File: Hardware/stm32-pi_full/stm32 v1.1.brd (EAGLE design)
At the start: 131.4 x 105.8 mm, 287 parts, among them J1 JUMPER-SMT_2_NC_TRACE_NO-SILK, Q1 PNP, Q2 NPN, Q3 NPN, U1 ESP32-WROOM-32D

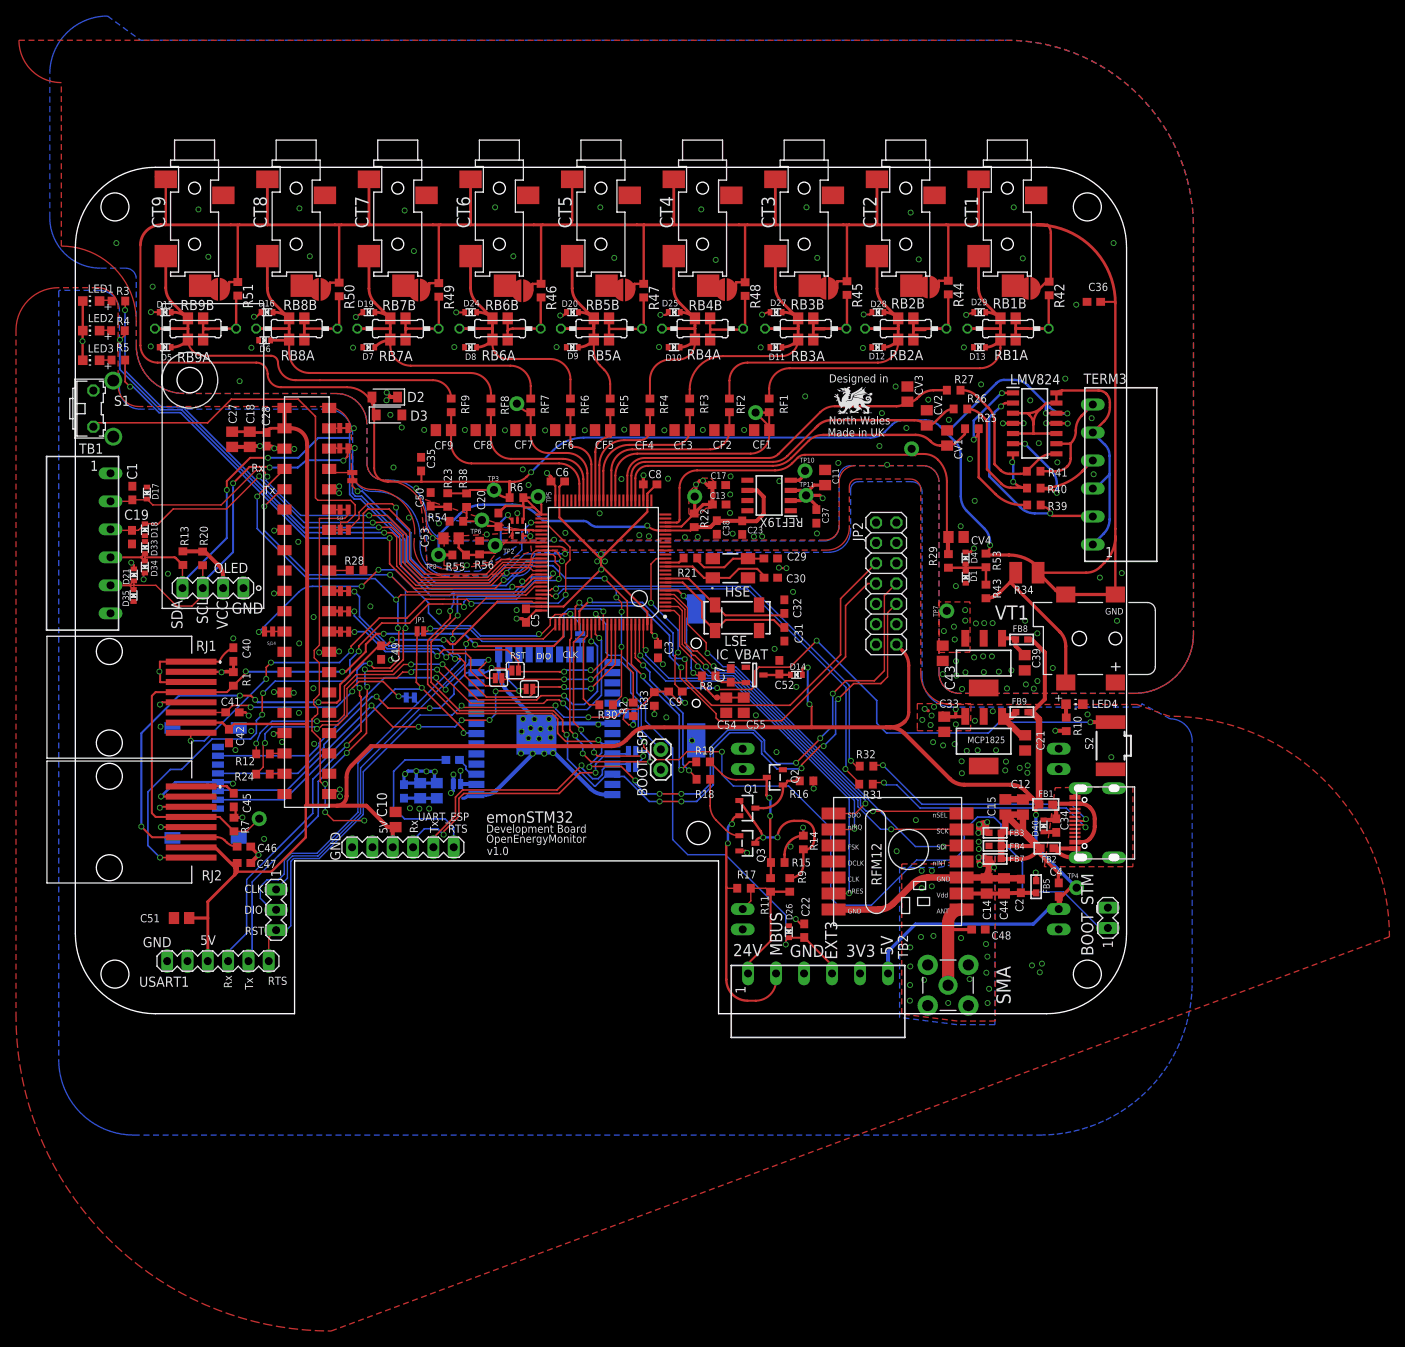
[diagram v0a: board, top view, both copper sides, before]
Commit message: tidy
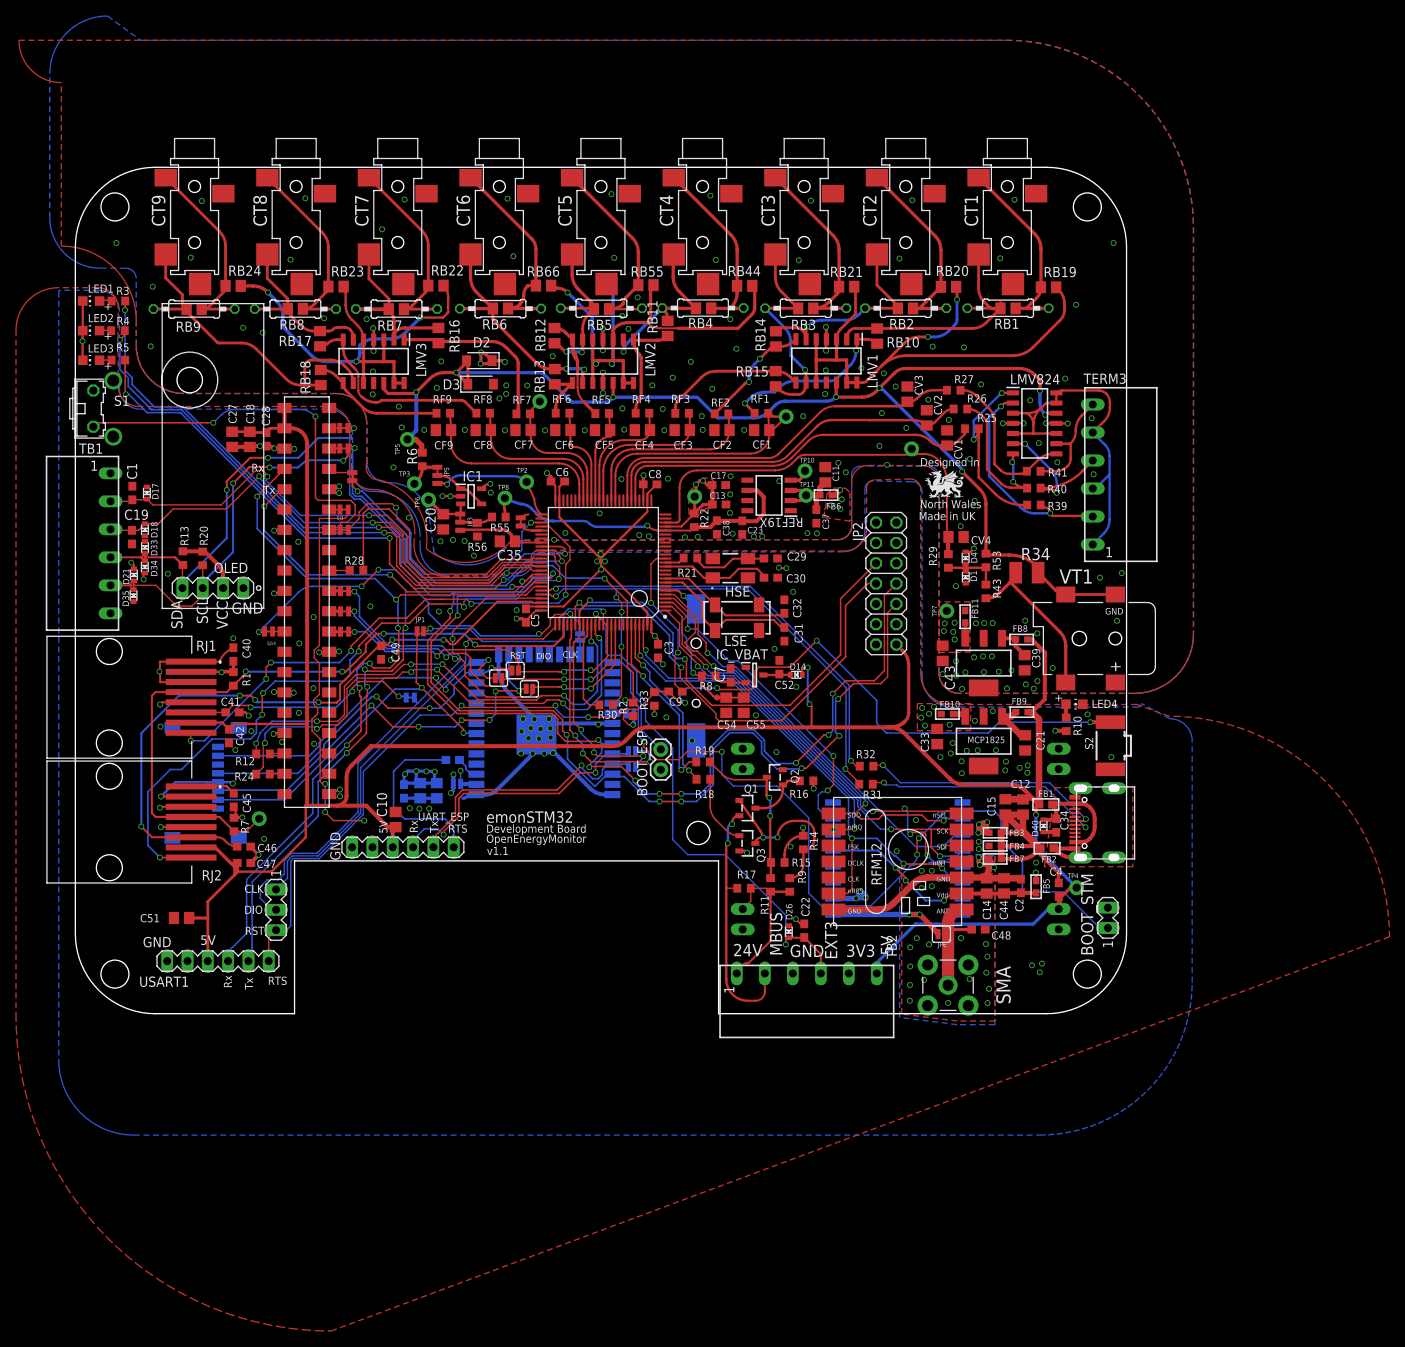
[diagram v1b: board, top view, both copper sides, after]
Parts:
- removed C36: (no value), rcl:C0603
- removed C50: 1uF, rcl:C0603
- removed C53: 22uF, rcl:C0805
- removed D10, D11, D12, D13, D15, D16, D19, D20, D24, D25, D27, D28, D29, D5, D6, D7, D8, D9: ESD5Z3.3T1G, microbuilder:SOD-523
- removed IC2: (no value), analog-devices:SC70-5
- removed JP10, JP11, JP12, JP13, JP14, JP15, JP16, JP17, JP18: JUMPER-SMT_2_NO_NO-SILK_ROUND, SparkFun-Jumpers:SMT-JUMPER_2_NO_NO-SILK_ROUND
- removed R23: 1k, resistor:R0603
- removed R38: 39k, resistor:R0603
- removed R42, R44, R45, R46, R47, R48, R49, R50, R51: 0R, rcl:R0603
- removed R54: 10k, resistor:R0603
- removed RB1A, RB2A, RB3A, RB4A, RB5A, RB6A, RB7A, RB8A, RB9A: 6R8, rcl:R0805
- removed RB1B, RB2B, RB3B, RB4B, RB5B, RB6B, RB7B, RB8B, RB9B: (no value), rcl:R0805
- added FB10, FB11, FB6: (no value), microbuilder:_0603
- added IC1: TS461CLT, TS461CLT:SOT95P280X145-5N
- added JP3, JP5: JUMPER-SMT_3_1-NC_TRACE_NO-SILK, SparkFun-Jumpers:SMT-JUMPER_3_1-NC_TRACE_NO-SILK
- added JP6: JUMPER-SMT_2_NC_PASTE_SILK, SparkFun-Jumpers:SMT-JUMPER_2_NC_PASTE_SILK
- added LMV1, LMV2, LMV3: LMV824IDG4, LMV824IDG4:SOIC127P600X175-14N
- added RB1, RB2, RB3, RB4, RB5, RB6, RB7, RB8, RB9: 6R81, rcl:R0805
- added RB10, RB11, RB12, RB13, RB14, RB15, RB16, RB17, RB18: 510R 0.1%, rcl:R0805
- added RB19, RB20, RB21, RB22, RB23, RB24, RB44, RB55, RB66: 680R | 681R 0.1%, rcl:R0805
- added SJ1: JUMPER-SMT_2_NC_TRACE_NO-SILK, SparkFun-Jumpers:SMT-JUMPER_2_NC_TRACE_NO-SILK
- added U2: RFM69HCW/RFM95W, microbuilder:RFMHCW_SMT
- C11, C23: value 1uF -> 22uf
- C20: value 2.2nF -> 22uF; device rcl:C0603 -> rcl:C0805
- C35: value (none) -> 22uF; device rcl:C0603 -> rcl:C0805
- FB1: value (none) -> 1600R
- FB2: value (none) -> 0R
- R55: value 91k -> 10k
- R6: value 0R -> 20R; device resistor:R0603 -> rcl:R0603
- moved TP5 17.8 mm to (41.5, 71.8)
- moved C35 14.5 mm to (54.0, 59.0), turned to 180 degrees
- moved R6 12.7 mm to (43.4, 69.3), turned to 90 degrees
- moved D2 12.7 mm to (50.5, 81.6)
- moved D3 12.1 mm to (50.7, 78.7)
- moved TP8 10.9 mm to (53.7, 64.5)
- moved TP3 9.98 mm to (42.4, 66.2)
- moved TP2 8.85 mm to (56.4, 66.5)
- moved TP6 7.12 mm to (44.2, 64.2)
- moved C20 6.90 mm to (46.0, 61.5), turned to 270 degrees
- moved R55 6.86 mm to (52.9, 62.1), turned to 0 degrees
- moved TP18 3.84 mm to (88.8, 74.6)
- moved TP19 2.88 mm to (58.1, 76.5)
- moved RB4_ 2.57 mm to (78.4, 88.2)
- moved RB1_ 2.54 mm to (116.6, 88.2)
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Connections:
- net CT1 renamed CT1_ADC
- net CT2 renamed CT2_ADC
- net CT3 renamed CT3_ADC
- net CT4 renamed CT4_ADC
- net CT5 renamed CT5_ADC
- net CT6 renamed CT6_ADC
- removed net OPAMP_NON-INVERT+: C53.1, IC2.3, R55.1, R56.2, STM32F303VE.58, TP2.1
- new net ANT_LORA: JP6.1, U2.1P
- new net BIAS123: LMV1.10, LMV1.13, LMV1.14, LMV1.3, LMV1.5, RB19.2, RB20.2, RB21.2
- new net BIAS456: LMV2.10, LMV2.13, LMV2.14, LMV2.3, LMV2.5, RB44.2, RB55.2, RB66.2
- new net BIAS789: LMV3.10, LMV3.13, LMV3.14, LMV3.3, LMV3.5, RB22.2, RB23.2, RB24.2
- new net BIAS_SOT23: IC1.1, IC1.4, JP5.2
- new net CT1_OUT: LMV1.1, RB10.1, RF1.1
- new net CT2_OUT: LMV1.7, RB14.1, RF2.1
- new net CT3_OUT: LMV1.8, RB15.2, RF3.1
- new net CT4_OUT: LMV2.1, RB11.1, RF4.1
- new net CT5_OUT: LMV2.7, RB12.1, RF5.1
- new net CT6_OUT: LMV2.8, RB13.2, RF6.1
- new net CT7_OUT: LMV3.1, RB16.1, RF7.1
- new net CT8_OUT: LMV3.7, RB17.1, RF8.1
- new net CT9_OUT: LMV3.8, RB18.2, RF9.1
- new net DIO1_RFM: STM32F303VE.3, U2.7P
- new net N$12: CT5.P$3
- new net N$38: CT4.P$3
- new net N$39: C20.1, IC1.3, JP3.3, TP6.1
- new net N$40: CT6.P$1, RB6.2, RB66.1, RB6_.2
- new net N$42: JP5.3, R6.1, TP3.1
- new net N$43: CT9.P$1, RB24.1, RB9.2, RB9_.2
- new net N$45: CT8.P$1, RB23.1, RB8.2, RB8_.2
- new net N$46: CT7.P$1, RB22.1, RB7.2, RB7_.2
- new net STM32_OPAMP_NON-INVERT+: C35.1, JP3.1, STM32F303VE.58
- new net STM32_OPAMP_OUT: JP5.1, STM32F303VE.51, TP2.1
- net +3V3: now also FB10.2; no longer MCP1825.3
- net +3V3ANA: now also FB11.2, FB6.2, IC1.2, LMV1.4, LMV2.4, LMV3.4; no longer C11.1, C37.1, D15.K, D16.K, D19.K, D20.K, D24.K, D25.K, D27.K, D28.K, D29.K, IC2.5, MCP1825(ANALOG).3, REF19X.2, REF19X.3, TP11.1
- net AGND: now also C20.2, IC1.5, LMV1.11, LMV2.11, LMV3.11; no longer C36.2, C50.2, C53.2, D10.A, D11.A, D12.A, D13.A, D5.A, D6.A, D7.A, D8.A, D9.A, IC2.2, R54.2
- net ANT: now also JP6.2
- net BIAS: now also LMV1.12, LMV2.12, LMV3.12, TP5.1; no longer C35.1, C36.1, CT1.P$1, CT2.P$1, CT3.P$1, CT4.P$1, CT5.P$1, CT6.P$1, CT7.P$1, CT8.P$1, CT9.P$1, JP10.1, JP11.1, JP12.1, JP13.1, JP14.1, JP15.1, JP16.1, JP17.1, JP18.1, R23.2, R38.1, R42.1, R44.1, R45.1, R46.1, R47.1, R48.1, R49.1, R50.1, R51.1, TP3.1
- net CT_IN1: now also LMV1.2, RB1.1, RB10.2; no longer D13.K, D29.A, RB1A.1, RB1B.1, RF1.1
- net CT_IN2: now also LMV1.6, RB14.2, RB2.1; no longer D12.K, D28.A, RB2A.1, RB2B.1, RF2.1
- net CT_IN3: now also LMV1.9, RB15.1, RB3.1; no longer D11.K, D27.A, RB3A.1, RB3B.1, RF3.1
- net CT_IN4: now also LMV2.2, RB11.2, RB4.1; no longer D10.K, D25.A, RB4A.1, RB4B.1, RF4.1
- net CT_IN5: now also LMV2.6, RB12.2, RB5.1; no longer D20.A, D9.K, RB5A.1, RB5B.1, RF5.1
- net CT_IN6: now also LMV2.9, RB13.1, RB6.1; no longer D24.A, D8.K, RB6A.1, RB6B.1, RF6.1
- net CT_IN7: now also LMV3.2, RB16.2, RB7.1; no longer D19.A, D7.K, RB7A.1, RB7B.1, RF7.1
- net CT_IN8: now also LMV3.6, RB17.2, RB8.1; no longer D16.A, D6.K, RB8A.1, RB8B.1, RF8.1
- net CT_IN9: now also LMV3.9, RB18.1, RB9.1; no longer D15.A, D5.K, RB9A.1, RB9B.1, RF9.1
- net DGND: now also U2.9P
- net DIO0_RFM: now also U2.6P
- net N$1: no longer JP10.2
- net N$10: no longer JP13.2
- net N$13: no longer JP14.2
- net N$2: no longer JP11.2
- net N$20: no longer JP15.2
- net N$21: no longer JP16.2
- net N$22: no longer JP17.2
- net N$23: no longer JP18.2
- net N$24: now also CT6.P$3; no longer R47.2, RB5A.2, RB5B.2, RB5_.2
- net N$25: now also FB10.1, MCP1825.3; no longer R46.2, RB6A.2, RB6B.2, RB6_.2
- net N$26: now also CT1.P$1, RB1.2, RB19.1; no longer R42.2, RB1A.2, RB1B.2
- net N$27: now also CT2.P$1, RB2.2, RB20.1; no longer R44.2, RB2A.2, RB2B.2
- net N$29: now also C11.1, C37.1, FB6.1, REF19X.2, REF19X.3, TP11.1; no longer R50.2, RB8A.2, RB8B.2, RB8_.2
- net N$34: now also FB11.1, MCP1825(ANALOG).3; no longer R51.2, RB9A.2, RB9B.2, RB9_.2
- net N$35: now also CT4.P$1, RB4.2, RB44.1; no longer R48.2, RB4A.2, RB4B.2
- net N$36: now also CT3.P$1, RB21.1, RB3.2, RB3_.2; no longer R49.2, RB7A.2, RB7B.2, RB7_.2
- net N$37: now also JP3.2, R55.1, R56.2; no longer R45.2, RB3A.2, RB3B.2, RB3_.2
- net N$7: now also CT5.P$1, RB5.2, RB55.1, RB5_.2; no longer C50.1, R23.1
- net N$8: no longer JP12.2
- net OPAMP_INVERT-: now also SJ1.1; no longer C20.1, IC2.4, R38.2, R54.1, TP6.1
- net OPAMP_OUT: now also SJ1.2; no longer C20.2, IC2.1, R6.1, STM32F303VE.51, TP5.1
- net RGND: now also U2.16P, U2.2P
- net RST_RFM: now also U2.14P
- net SPI4_CLK_MASTER: now also U2.12P
- net SPI4_CS_RFM69_MASTER: now also U2.13P
- net SPI4_MISO_MASTER: now also U2.10P
- net SPI4_MOSI_MASTER: now also U2.11P
- net VDD: now also U2.5P
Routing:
- net BIAS: track 525.0 -> 159.3 mm, vias 4 -> 8
- net BIAS123: track 0.00 -> 71.8 mm, vias 0 -> 2
- net BIAS456: track 0.00 -> 68.0 mm, vias 0 -> 3
- net BIAS789: track 0.00 -> 61.6 mm, vias 0 -> 3
- net DIO1_RFM: track 0.00 -> 39.9 mm, vias 0 -> 3
- net +3V3ANA: track 73.2 -> 40.1 mm, vias 23 -> 25
- net CT_IN8: track 49.6 -> 22.5 mm
- net N$40: track 0.00 -> 26.0 mm
- net CT8_OUT: track 0.00 -> 26.0 mm
- net N$45: track 0.00 -> 25.2 mm
- net N$43: track 0.00 -> 25.0 mm
- net N$46: track 0.00 -> 24.9 mm
- net N$7: track 2.18 -> 25.9 mm
- net CT1_OUT: track 0.00 -> 22.5 mm, vias 0 -> 2
- net CT7_OUT: track 0.00 -> 22.4 mm
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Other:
- board text added: "v1.1"
- board text removed: "v1.0"
